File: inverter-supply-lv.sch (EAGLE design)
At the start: 64 parts, among them IC1 1039-2387**3.3V 300mA LDO Vol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, U1 1039-2397** MP2456GJ-Z 0.5A, 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, U2 1039-9015**AOZ1282CI Buck Swi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, X1 0289-9066**15EDGVC-3.81-02P-14

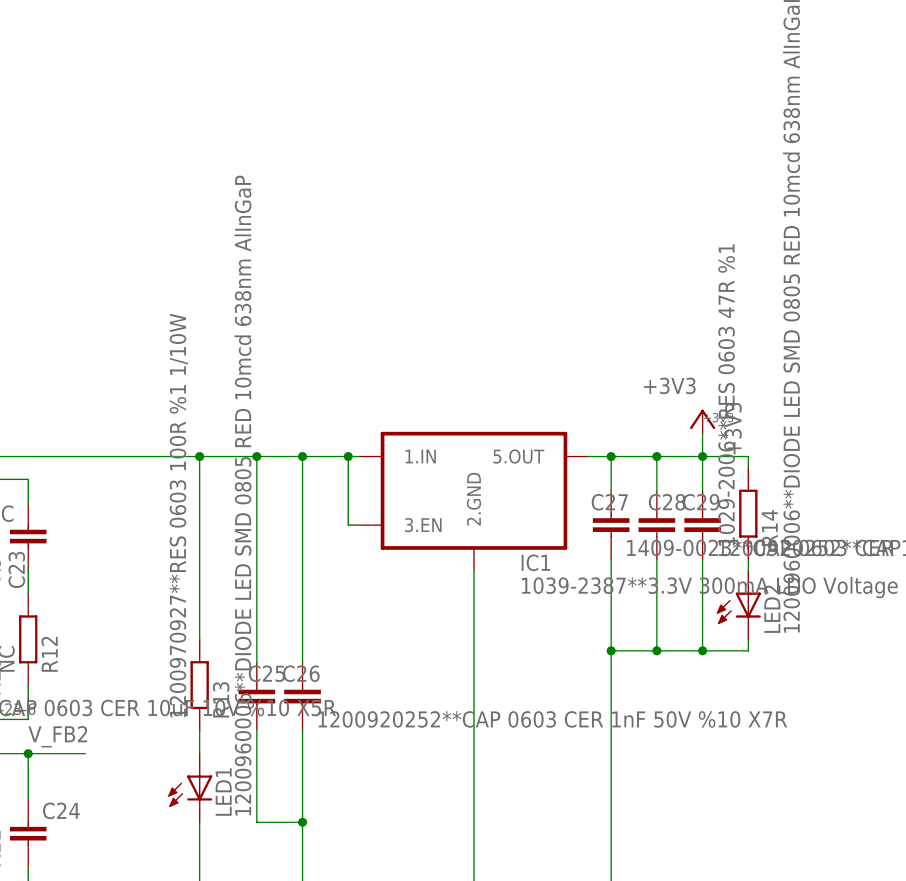
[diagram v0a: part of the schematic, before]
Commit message: Malzeme degerlerinde degisiklikler yapilmisti sanirim.
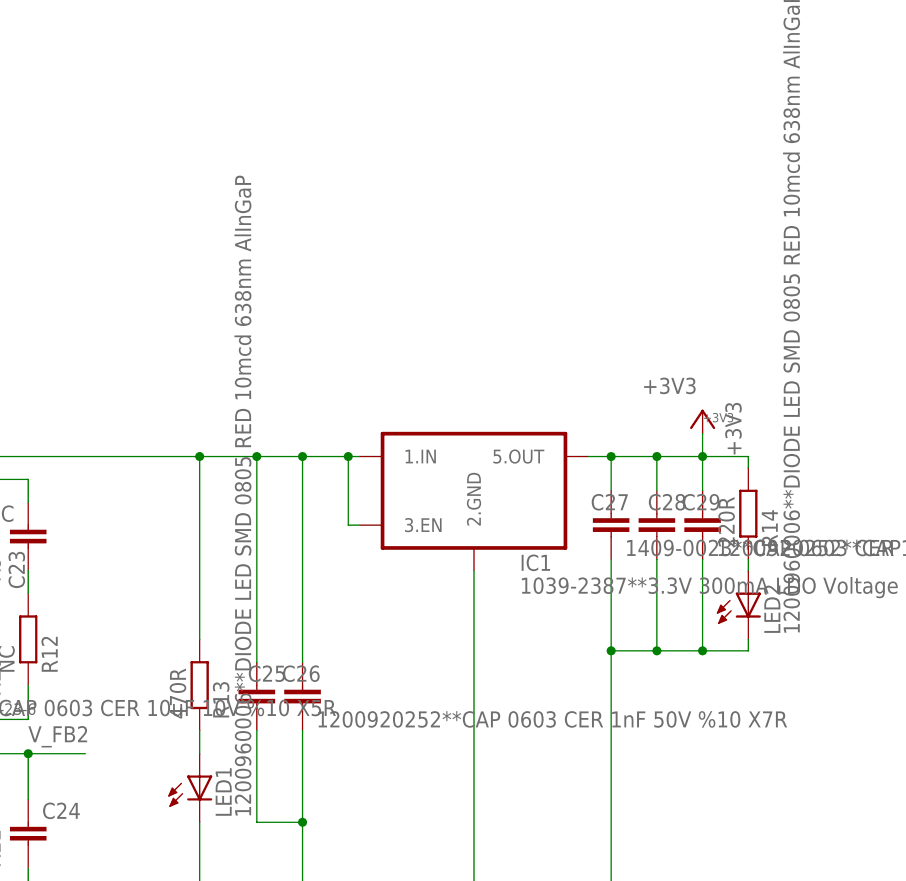
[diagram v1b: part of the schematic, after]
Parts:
- R13: value 1200970927**RES 0603 100R %1 1/10W -> 470R
- R14: value 1029-2006**RES 0603 47R %1 -> 220R
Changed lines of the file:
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@@
 <part name="C10" library="rcl" deviceset="C-EU" device="C0603E" value="1200920268**CAP 0603 CER 100nF 50V %10 X7R"/>
 <part name="LED1" library="led" deviceset="LED" device="CHIP-LED0805" value="1200960006**DIODE LED SMD 0805 RED 10mcd 638nm AlInGaP"/>
-<part name="R13" library="rcl" deviceset="R-EU_" device="R0603E" value="1200970927**RES 0603 100R %1 1/10W"/>
+<part name="R13" library="rcl" deviceset="R-EU_" device="R0603E" value="470R"/>
 <part name="IC1" library="enko" deviceset="NCP115ASN330T2G" device="" value="1039-2387**3.3V 300mA LDO Voltage Regulator TSOP-5"/>
 <part name="C18" library="rcl" deviceset="C-EU" device="C0603E" value="1200920268**CAP 0603 CER 100nF 50V %10 X7R"/>
@@
 <part name="C19" library="rcl" deviceset="C-EU" device="C0603E" value="1200920252**CAP 0603 CER 1nF 50V %10 X7R"/>
 <part name="C21" library="rcl" deviceset="C-EU" device="C0603E" value="1019-3387**CAP 0603 CER 10uF 10V %10 X5R"/>
-<part name="R14" library="rcl" deviceset="R-EU_" device="R0603E" value="1029-2006**RES 0603 47R %1"/>
+<part name="R14" library="rcl" deviceset="R-EU_" device="R0603E" value="220R"/>
 <part name="LED2" library="led" deviceset="LED" device="CHIP-LED0805" value="1200960006**DIODE LED SMD 0805 RED 10mcd 638nm AlInGaP"/>
 <part name="C11" library="rcl" deviceset="C-EU" device="C0805E" value="10uF 50V %10 X7R"/>
